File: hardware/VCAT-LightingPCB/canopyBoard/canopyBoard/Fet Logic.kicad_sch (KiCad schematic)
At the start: 3 parts

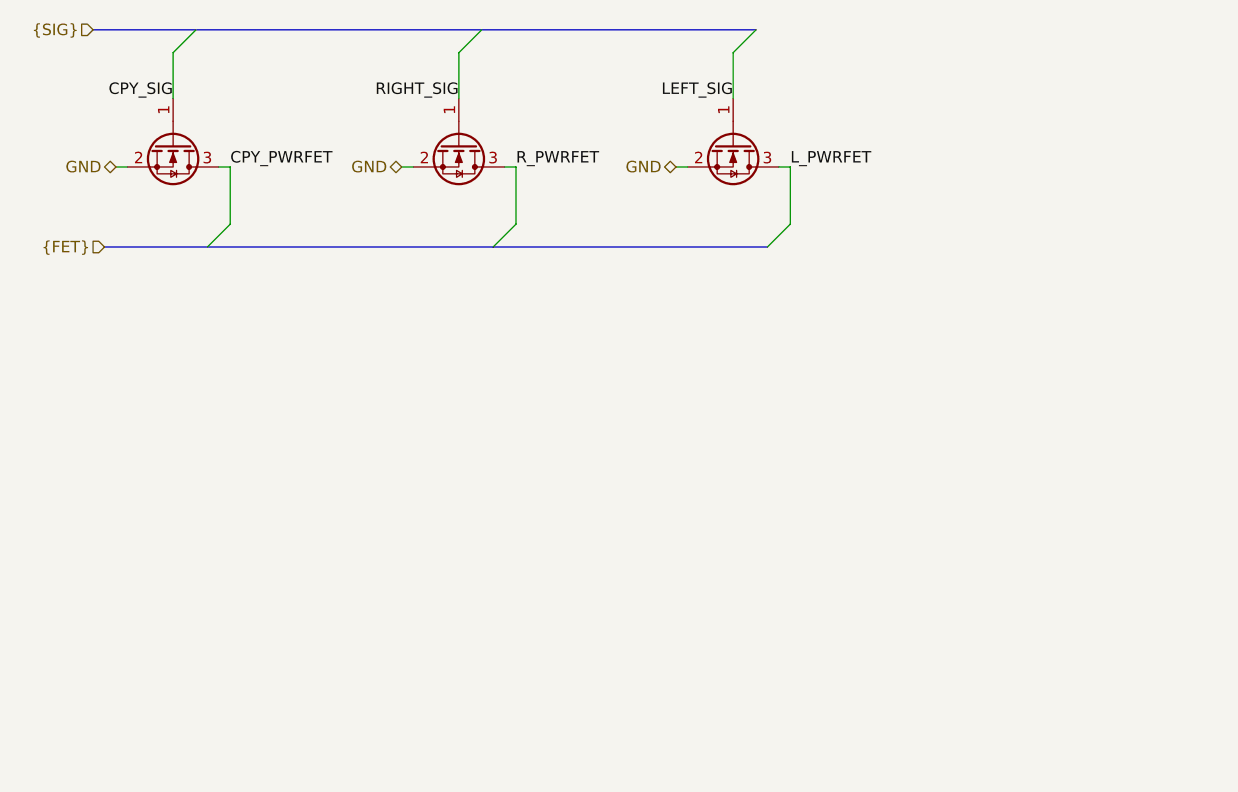
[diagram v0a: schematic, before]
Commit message: pray for no errors, more stuff to add
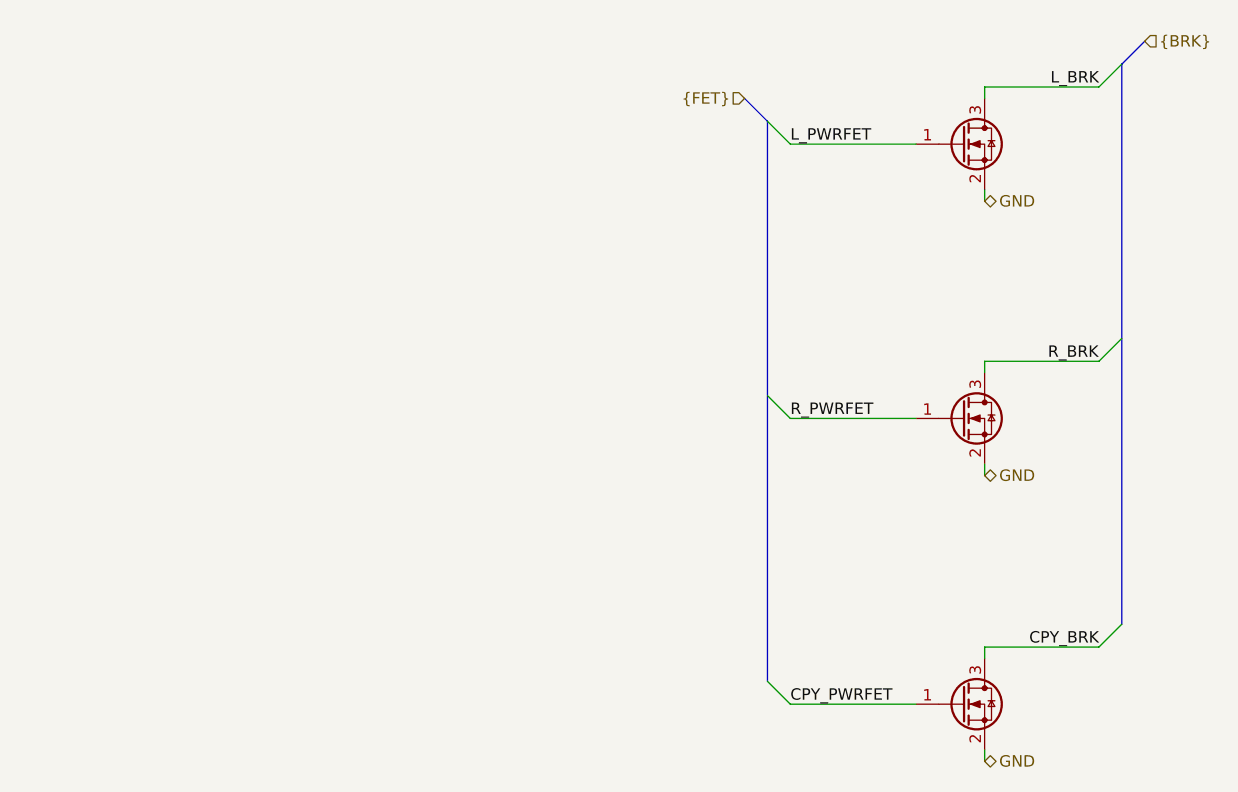
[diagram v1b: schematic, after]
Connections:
- net CPY_SIG is gone; now on net CPY_PWRFET: IRLML0030TRPBF7.1 (G)
- net LEFT_SIG is gone; now on net L_PWRFET: IRLML0030TRPBF5.1 (G)
- net RIGHT_SIG is gone; now on net R_PWRFET: IRLML0030TRPBF6.1 (G)
- net CPY_PWRFET: no longer IRLML0030TRPBF7.3 (D)
- net L_PWRFET: no longer IRLML0030TRPBF5.3 (D)
- net R_PWRFET: no longer IRLML0030TRPBF6.3 (D)
- new net CPY_BRK: IRLML0030TRPBF7.3 (D)
- new net L_BRK: IRLML0030TRPBF5.3 (D)
- new net R_BRK: IRLML0030TRPBF6.3 (D)
